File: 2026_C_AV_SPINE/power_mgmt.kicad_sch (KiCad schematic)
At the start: 74 parts, among them Q1 PMOS, Q2 PMOS, Q3 PMOS, Q4 PMOS, Q5 NMOS, Q6 NMOS, Q7 NMOS, Q8 NMOS, U3 LTC4418IUF_TRPBF, U4 LM5176RHF

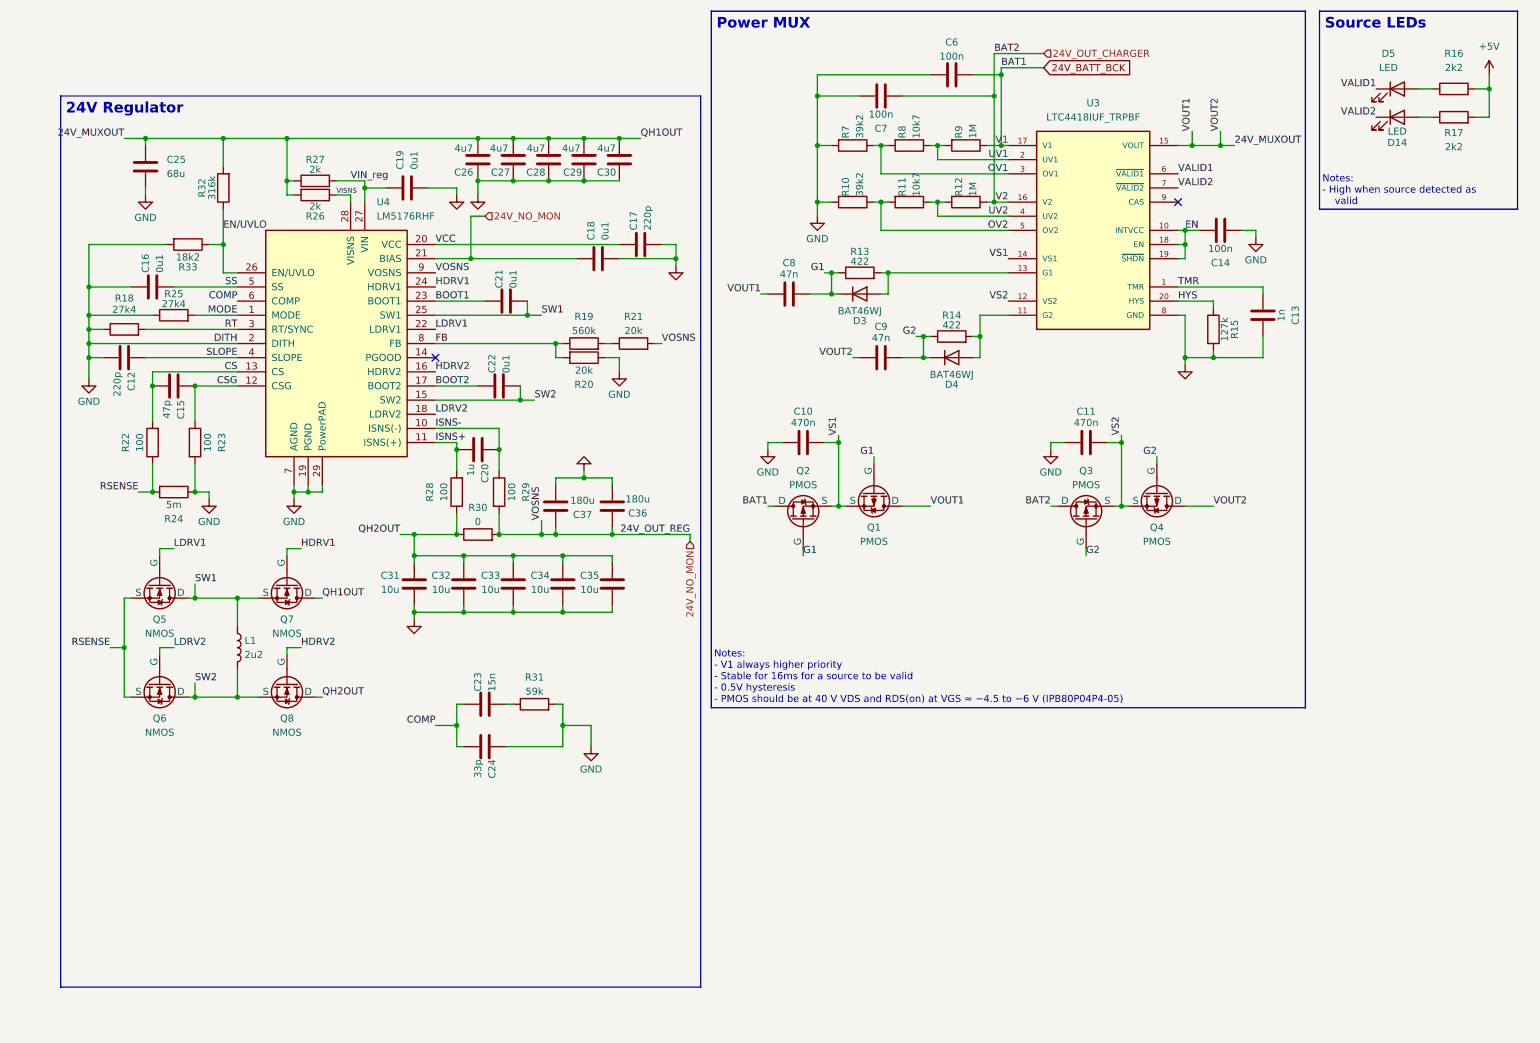
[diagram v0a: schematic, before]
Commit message: spine almost finished
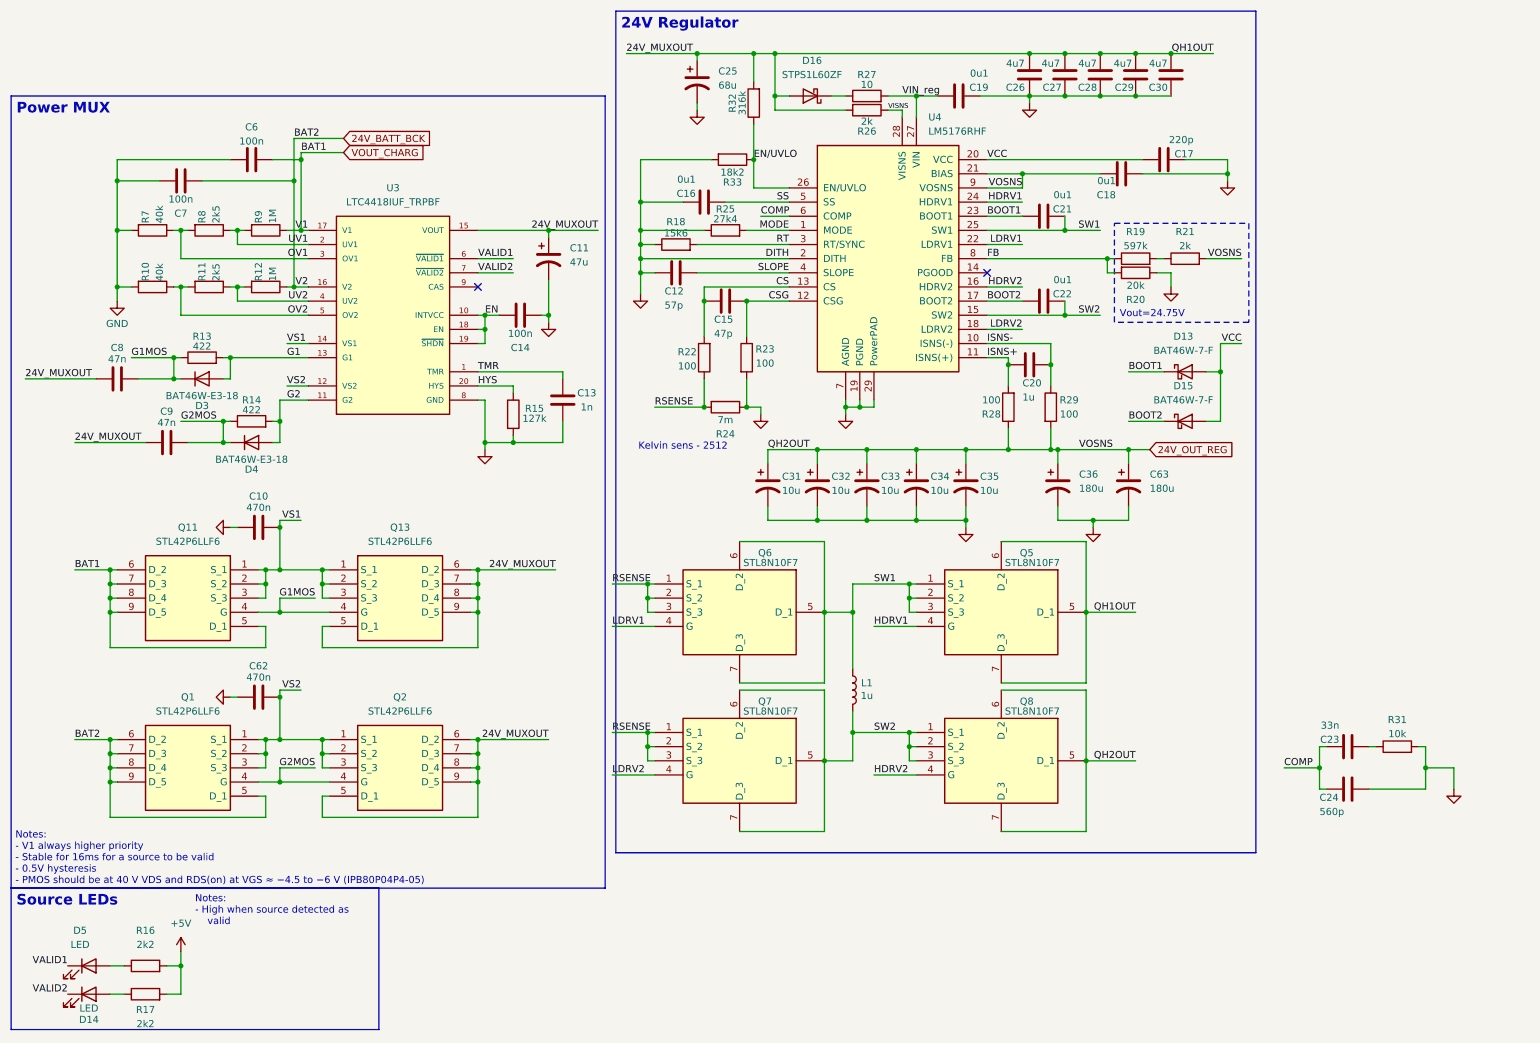
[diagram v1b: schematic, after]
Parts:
- removed C11: 470n, Capacitor_SMD:C_0603_1608Metric, symbol Device:C
- removed C25: 68u, Capacitor_SMD:C_Elec_5x5.8, symbol Device:C
- removed C31, C32, C33, C34, C35: 10u, Capacitor_SMD:C_Elec_4x5.4, symbol Device:C
- removed C36, C37: 180u, Capacitor_SMD:C_Elec_6.3x7.7, symbol Device:C
- removed Q1, Q2, Q3, Q4: PMOS, Package_SO:PowerPAK_SO-8_Single, symbol Simulation_SPICE:PMOS
- removed Q5, Q6, Q7, Q8: NMOS, Package_TO_SOT_SMD:LFPAK33, symbol Simulation_SPICE:NMOS
- removed R30: 0, Resistor_SMD:R_0603_1608Metric, symbol Device:R
- added C11: 47u, Capacitor_SMD:CP_Elec_6.3x9.9, symbol Device:C_Polarized_US
- added C25: 68u, Capacitor_SMD:CP_Elec_6.3x5.9, symbol Device:C_Polarized_US
- added C31, C32, C33, C34, C35: 10u, Capacitor_SMD:C_Elec_4x5.4, symbol Device:C_Polarized_US
- added C36, C63: 180u, Capacitor_SMD:CP_Elec_10x10.5, symbol Device:C_Polarized_US
- added C62: 470n, Capacitor_SMD:C_0603_1608Metric, symbol Device:C
- added D13, D15: BAT46W-7-F, Diode_SMD:D_SOD-123, symbol Diode:BAT46
- added D16: STPS1L60ZF, Diode_SMD:D_SOD-123, symbol Diode:BAT46
- added Q1, Q11, Q13, Q2: STL42P6LLF6, ert:STL42P6LLF6, symbol ert:STL42P6LLF6
- added Q5, Q6, Q7, Q8: STL8N10F7, ert:STL8N10F7, symbol ert:STL8N10F7
- C12: value 220p -> 57p
- C23: value 15n -> 33n
- C24: value 33p -> 560p
- D3, D4: value BAT46WJ -> BAT46W-E3-18; footprint (none) -> Diode_SMD:D_SOD-123; Mouser (none) -> https://www.mouser.ch/ProductDetail/Vishay-Semiconductors/B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
- L1: value 2u2 -> 1u; footprint Inductor_SMD:L_0603_1608Metric -> Inductor_SMD:L_10.4x10.4_H4.8; Mouser (none) -> https://www.mouser.ch/ProductDetail/KEMET/MPX1D1040L1R0?qs=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; no (none) -> MPX1D1040L1R0
- R10, R7: value 39k2 -> 40k
- R11, R8: value 10k7 -> 2k5
- R18: value 27k4 -> 15k6
- R19: value 560k -> 597k; Mouser (none) -> https://www.mouser.ch/ProductDetail/YAGEO/RT0603BRD07597KL?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
- R21: value 20k -> 2k
- R24: value 5m -> 7m; footprint Resistor_SMD:R_0603_1608Metric -> Resistor_SMD:R_2512_6332Metric
- R27: value 2k -> 10
- R31: value 59k -> 10k
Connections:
- net 24V_OUT_CHARGER is gone; now on net 24V_BATT_BCK: C7.1, R12.1, U3.16 (V2)
- net QH2OUT is gone; now on net 24V_OUT_REG: R28.1
- net 24V_BATT_BCK: now also Q1.5 (D_1), Q1.6 (D_2), Q1.7 (D_3), Q1.8 (D_4), Q1.9 (D_5); no longer C6.2, R9.1, U3.17 (V1)
- net 24V_MUXOUT: now also C11.1, C25.1, D16.2 (A), Q13.5 (D_1), Q13.6 (D_2), Q13.7 (D_3), Q13.8 (D_4), Q13.9 (D_5), Q2.5 (D_1), Q2.6 (D_2), Q2.7 (D_3), Q2.8 (D_4), Q2.9 (D_5), Q5.5 (D_1), Q5.6 (D_2), Q5.7 (D_3); no longer R27.1
- net BOOT1: now also D13.1 (K)
- net BOOT2: now also D15.1 (K)
- net G1: now also D3.2 (A), R13.2, U3.13 (G1); no longer C8.2, D3.1 (K), R13.1
- net G2: now also D4.2 (A), R14.2, U3.11 (G2); no longer C9.2, D4.1 (K), R14.1
- net GND: now also C11.2, C25.2, C31.2, C32.2, C33.2, C34.2, C35.2, C36.2, C62.1, C63.2
- net HDRV1: now also Q5.4 (G)
- net HDRV2: now also Q8.4 (G)
- net LDRV1: now also Q6.4 (G)
- net LDRV2: now also Q7.4 (G)
- net RSENSE: now also Q6.1 (S_1), Q6.2 (S_2), Q6.3 (S_3), Q7.1 (S_1), Q7.2 (S_2), Q7.3 (S_3)
- net SW1: now also Q5.1 (S_1), Q5.2 (S_2), Q5.3 (S_3), Q6.5 (D_1), Q6.6 (D_2), Q6.7 (D_3)
- net SW2: now also Q7.5 (D_1), Q7.6 (D_2), Q7.7 (D_3), Q8.1 (S_1), Q8.2 (S_2), Q8.3 (S_3)
- net VCC: now also D13.2 (A), D15.2 (A)
- net VS1: now also Q11.1 (S_1), Q11.2 (S_2), Q11.3 (S_3), Q13.1 (S_1), Q13.2 (S_2), Q13.3 (S_3)
- net VS2: now also C62.2, Q1.1 (S_1), Q1.2 (S_2), Q1.3 (S_3), Q2.1 (S_1), Q2.2 (S_2), Q2.3 (S_3)
- net 24V_NO_MON renamed 24V_OUT_REG
- net 24V_OUT_REG: now also C31.1, C32.1, C33.1, C34.1, C35.1, C36.1, C63.1, Q8.5 (D_1), Q8.6 (D_2), Q8.7 (D_3)
- new net: D16.1 (K), R27.1
- new net G1MOS: C8.2, D3.1 (K), Q11.4 (G), Q13.4 (G), R13.1
- new net G2MOS: C9.2, D4.1 (K), Q1.4 (G), Q2.4 (G), R14.1
- new net VOUT_CHARG: C6.2, Q11.5 (D_1), Q11.6 (D_2), Q11.7 (D_3), Q11.8 (D_4), Q11.9 (D_5), R9.1, U3.17 (V1)
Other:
- note added: "Kelvin sens - 2512"
- moved on the sheet: C10, C12, C13, C14, C15, C16, C17, C18, C19, C20, C21, C22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
